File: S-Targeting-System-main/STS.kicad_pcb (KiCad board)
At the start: 2 copper layers, 56 x 56 mm, 18 parts, among them J1 Conn_01x01_Pin, J2 Conn_01x01_Pin, M1 Motor_Servo, M2 Motor_Servo, M3 Motor_Servo, U1 ADG633YCP, U2 BMP180, U3 SD_Card_Reader, U4 MPU, U6 HC-12

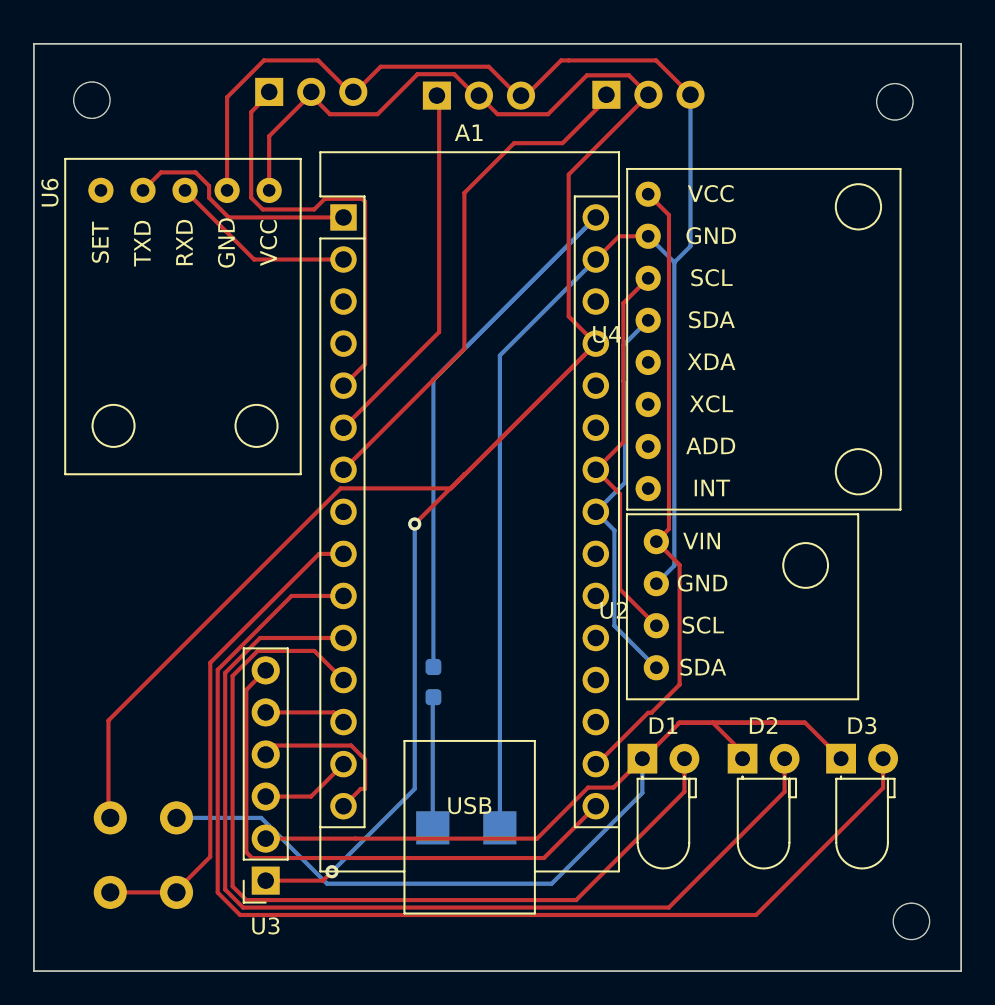
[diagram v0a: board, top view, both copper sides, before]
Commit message: 40x60
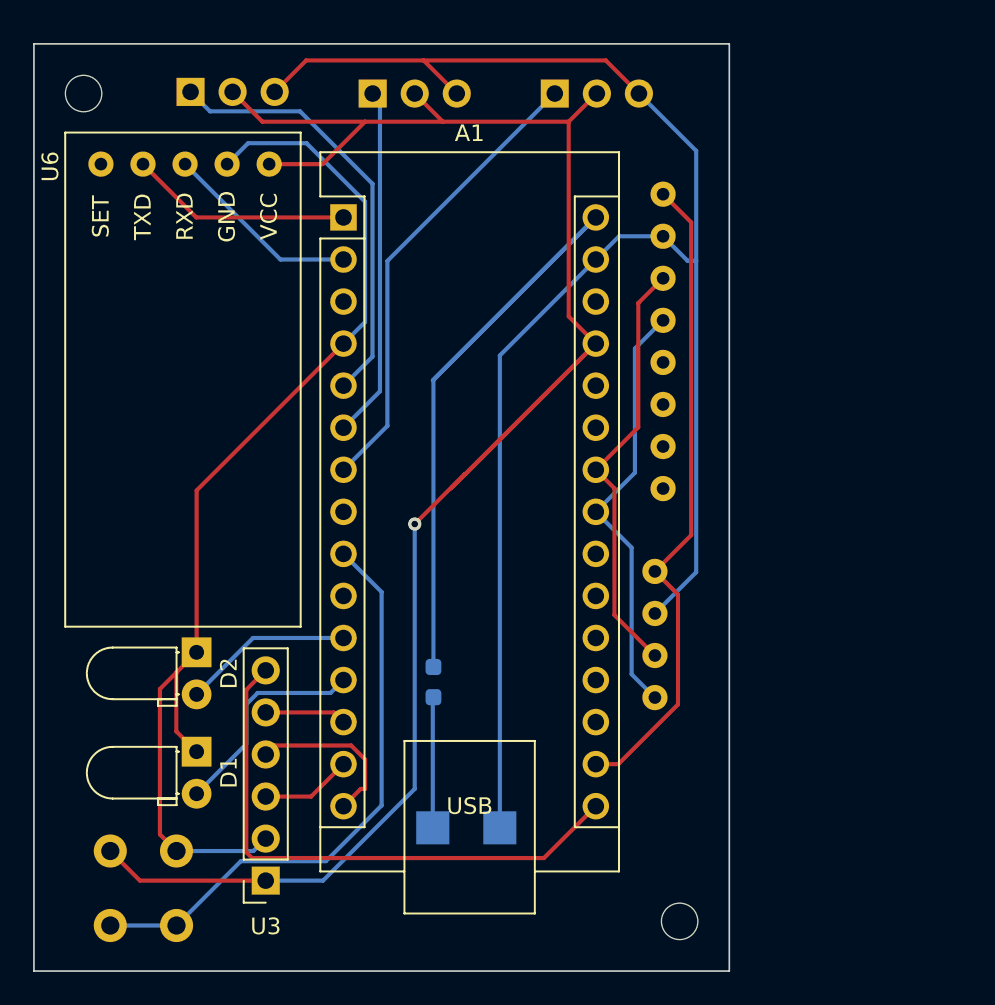
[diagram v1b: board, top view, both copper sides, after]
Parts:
- removed D3: LED, LED_THT:LED_D3.0mm_Horizontal_O1.27mm_Z2.0mm
- removed the REF** at (102.5, 64.4)
- U2, U4: moved to B.Cu
- moved REF** 49.0 mm to (102.0, 64.0)
- moved D2 33.6 mm to (108.8, 97.8), turned to -90 degrees
- moved D1 26.9 mm to (108.8, 103.8), turned to -90 degrees
- moved REF** 14.0 mm to (138.0, 114.0)
- moved M2 4.75 mm to (108.4, 63.9)
- moved M3 3.88 mm to (119.4, 64.0)
- moved M1 3.12 mm to (130.5, 64.0)
- moved U1 2.00 mm to (101.1, 109.8)
- moved U2 1.80 mm to (136.5, 100.5), turned to 180 degrees
- moved U6 1.59 mm to (103.0, 68.3)
- moved U4 0.90 mm to (137.0, 87.9), turned to 180 degrees
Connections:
- J2 pad 1: Net-(J2-Pin_1) -> Earth
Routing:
- net /D7: track 68.6 -> 0.00 mm
- net /D8: track 60.2 -> 10.3 mm
- net /D9: track 53.1 -> 13.1 mm
- net Net-(J2-Pin_1): track 36.7 -> 0.00 mm
- net /5V: track 136.6 -> 112.0 mm, vias 2 -> 1
- net Earth: track 157.9 -> 170.4 mm
- net /D6: track 29.5 -> 35.5 mm
- net /D4: track 30.9 -> 28.0 mm
- net Net-(A1-A5): track 23.8 -> 25.9 mm
- net Net-(A1-A4): track 23.9 -> 25.9 mm
- net Net-(A1-3V3): track 38.1 -> 39.5 mm
- net /D3: track 22.6 -> 21.3 mm
- net /TX: track 14.1 -> 13.4 mm
- net /RX: track 11.3 -> 12.0 mm
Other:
- board size 56 x 56 mm -> 42 x 56 mm

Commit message: final
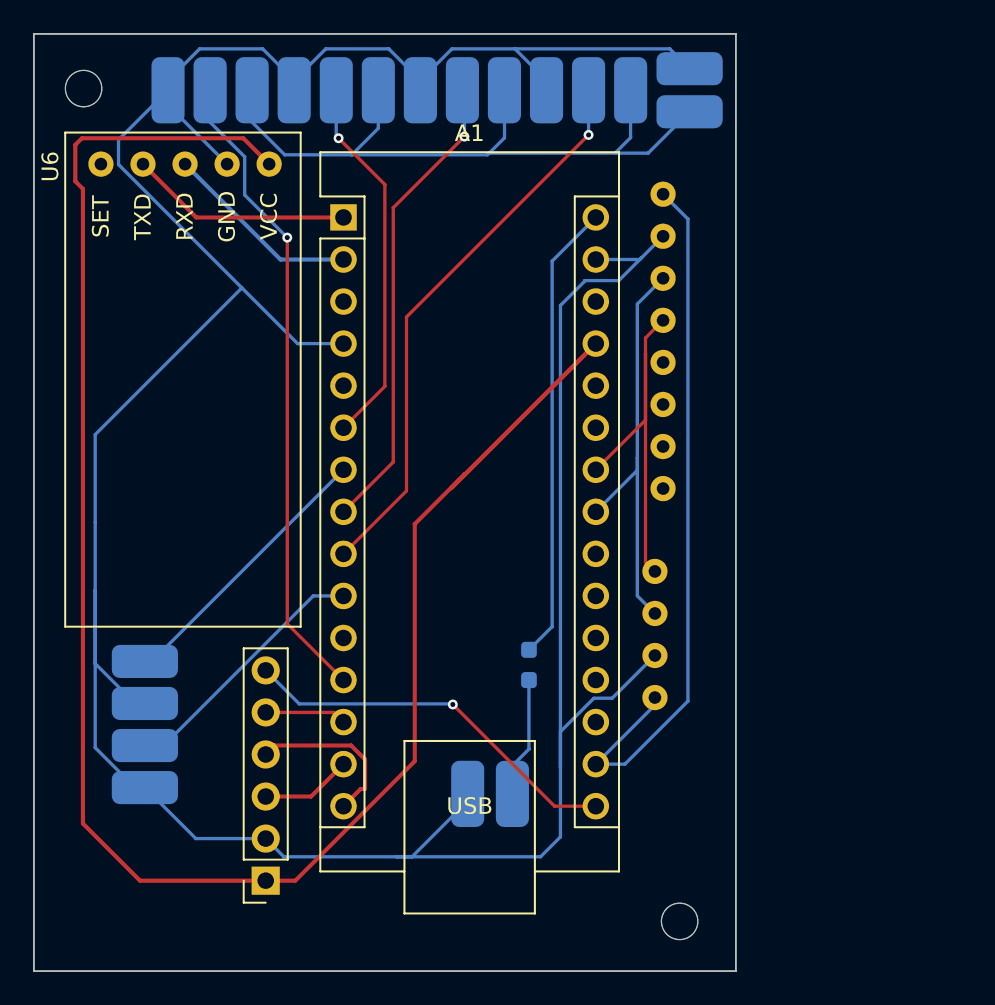
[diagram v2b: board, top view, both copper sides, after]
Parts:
- removed D1, D2: LED, LED_THT:LED_D3.0mm_Horizontal_O1.27mm_Z2.0mm
- removed J1, J2: Conn_01x01_Pin, TestPoint:TestPoint_Pad_2.0x2.0mm
- removed M1, M2, M3: Motor_Servo, Connector_PinHeader_2.54mm:PinHeader_1x03_P2.54mm_Horizontal
- removed U1: ADG633YCP, Button_Switch_THT:SW_PUSH_6mm_H4.3mm
- added ?: , , F.Cu at (125.2, 106.3)
- added ?: , , F.Cu at (127.9, 106.3)
- added ?: , , F.Cu at (138.6, 65.1)
- added ?: , , F.Cu at (138.6, 62.5)
- added GND: SolderWirePad_1x01_SMD_1x2mm, Connector_Wire:SolderWirePad_1x01_SMD_1x2mm, B.Cu at (105.7, 100.8)
- added GND: SolderWirePad_1x01_SMD_1x2mm, Connector_Wire:SolderWirePad_1x01_SMD_1x2mm, B.Cu at (105.7, 105.9)
- added L1: SolderWirePad_1x01_SMD_1x2mm, Connector_Wire:SolderWirePad_1x01_SMD_1x2mm, B.Cu at (105.7, 103.4)
- added L2: L2, , B.Cu at (105.7, 98.3)
- added REF**: SolderWirePad_1x01_SMD_1x2mm, Connector_Wire:SolderWirePad_1x01_SMD_1x2mm, B.Cu at (135.0, 63.8)
- added REF**1: SolderWirePad_1x01_SMD_1x2mm, Connector_Wire:SolderWirePad_1x01_SMD_1x2mm, B.Cu at (132.5, 63.8)
- added REF**10: SolderWirePad_1x01_SMD_1x2mm, Connector_Wire:SolderWirePad_1x01_SMD_1x2mm, B.Cu at (109.6, 63.8)
- added REF**11: SolderWirePad_1x01_SMD_1x2mm, Connector_Wire:SolderWirePad_1x01_SMD_1x2mm, B.Cu at (107.1, 63.8)
- added REF**2: SolderWirePad_1x01_SMD_1x2mm, Connector_Wire:SolderWirePad_1x01_SMD_1x2mm, B.Cu at (130.0, 63.8)
- added REF**3: SolderWirePad_1x01_SMD_1x2mm, Connector_Wire:SolderWirePad_1x01_SMD_1x2mm, B.Cu at (127.4, 63.8)
- added REF**4: SolderWirePad_1x01_SMD_1x2mm, Connector_Wire:SolderWirePad_1x01_SMD_1x2mm, B.Cu at (124.9, 63.8)
- added REF**5: SolderWirePad_1x01_SMD_1x2mm, Connector_Wire:SolderWirePad_1x01_SMD_1x2mm, B.Cu at (122.3, 63.8)
- added REF**6: SolderWirePad_1x01_SMD_1x2mm, Connector_Wire:SolderWirePad_1x01_SMD_1x2mm, B.Cu at (119.8, 63.8)
- added REF**7: SolderWirePad_1x01_SMD_1x2mm, Connector_Wire:SolderWirePad_1x01_SMD_1x2mm, B.Cu at (117.3, 63.8)
- added REF**8: SolderWirePad_1x01_SMD_1x2mm, Connector_Wire:SolderWirePad_1x01_SMD_1x2mm, B.Cu at (114.7, 63.8)
- added REF**9: SolderWirePad_1x01_SMD_1x2mm, Connector_Wire:SolderWirePad_1x01_SMD_1x2mm, B.Cu at (112.2, 63.8)
- U4: value MPU -> module_mpu6050
- moved R1 5.86 mm to (128.9, 98.5)
- moved REF** 0.30 mm to (102.0, 63.7)
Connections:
- A1 pad 8: unconnected-(A1-D5-Pad8) -> /D5
- U2 pad 1: Net-(A1-3V3) -> Net-(A1-A5)
- U2 pad 2: Earth -> Net-(A1-A4)
- U2 pad 3: Net-(A1-A5) -> Earth
- U2 pad 4: Net-(A1-A4) -> Net-(A1-3V3)
- U4 pad 3: Net-(A1-A5) -> Net-(A1-A4)
- U4 pad 4: Net-(A1-A4) -> Net-(A1-A5)
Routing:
- net (no net): track 0.00 -> 43.2 mm
- net Earth: track 170.4 -> 200.7 mm
- net /D5: track 0.00 -> 28.5 mm, vias 0 -> 1
- net /D2: track 26.2 -> 0.00 mm
- net /D9: track 13.1 -> 39.0 mm, vias 0 -> 1
- net Net-(A1-VIN): track 45.1 -> 27.8 mm
- net /D7: track 0.00 -> 15.7 mm
- net /D4: track 28.0 -> 16.8 mm
- net /D13: track 34.0 -> 23.3 mm, vias 0 -> 1
- net /D8: track 10.3 -> 0.00 mm
- net /5V: track 112.0 -> 120.3 mm, vias 1 -> 0
- net Net-(A1-3V3): track 39.5 -> 43.9 mm
- net Net-(A1-A5): track 25.9 -> 24.1 mm
- net /D6: track 35.5 -> 34.1 mm, vias 0 -> 1
- net /D3: track 21.3 -> 22.6 mm, vias 0 -> 1
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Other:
- board size 42 x 56 mm -> 42.4 x 56.6 mm
